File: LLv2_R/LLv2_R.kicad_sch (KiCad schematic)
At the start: 12 parts, among them J1 AudioJack4

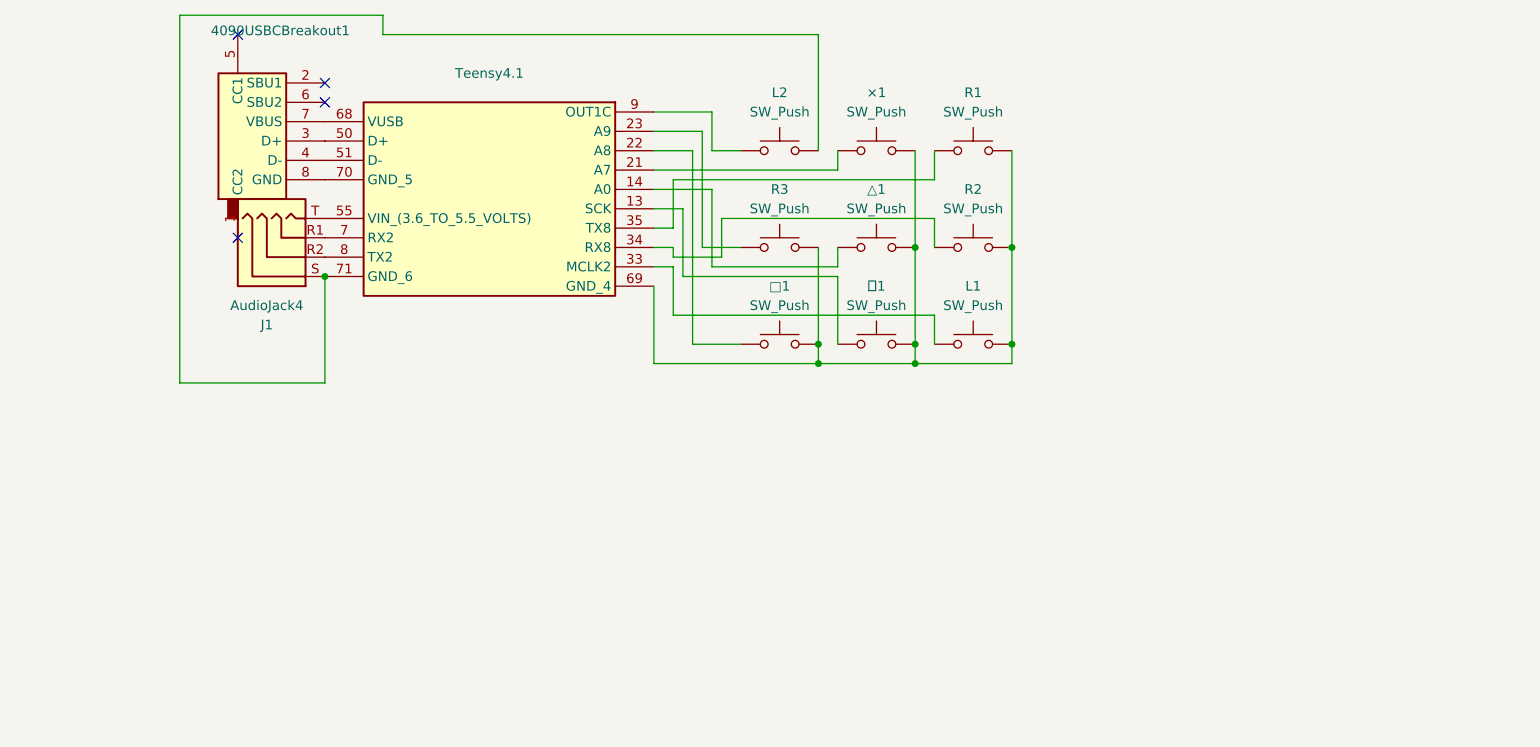
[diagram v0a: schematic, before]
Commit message: Update Softwere
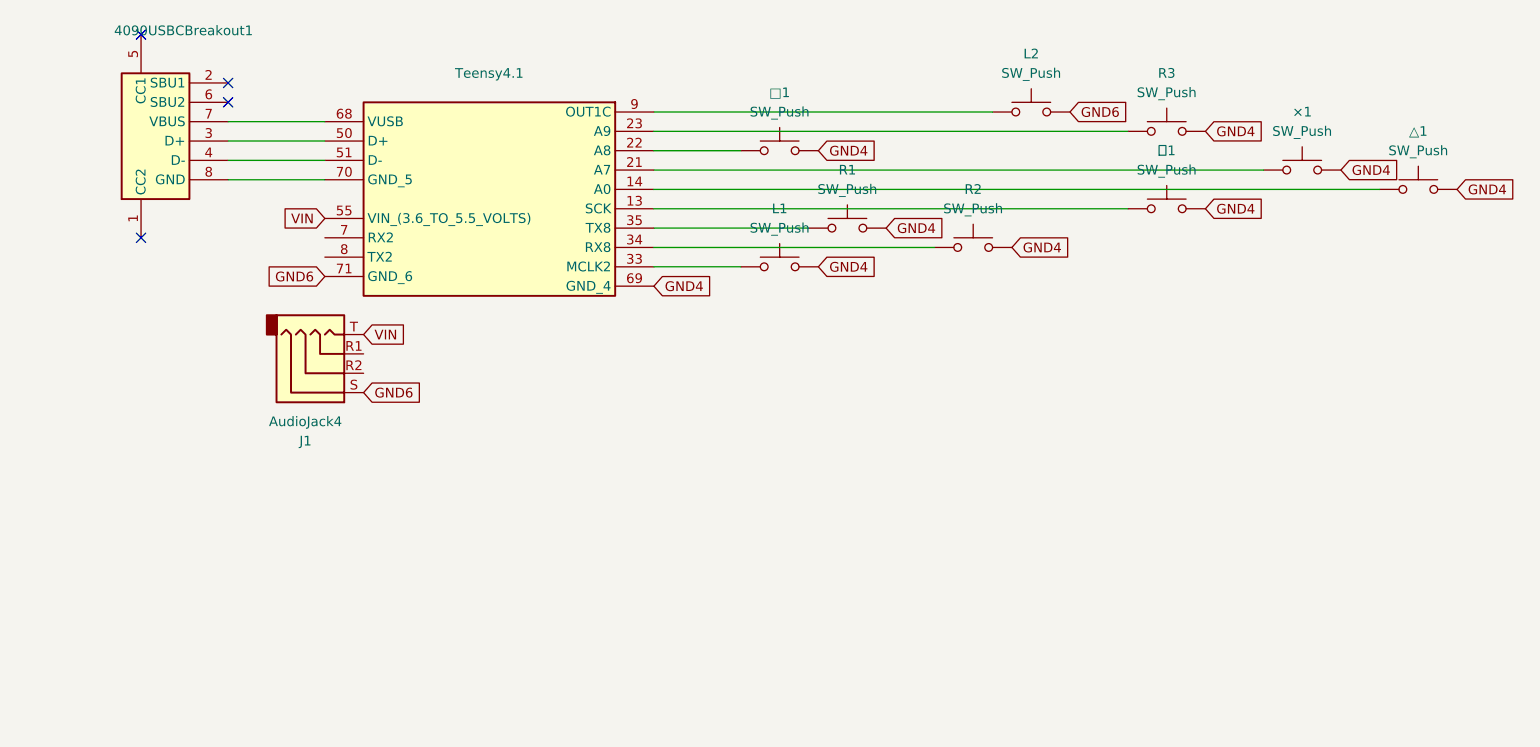
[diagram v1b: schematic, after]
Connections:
- net GND4: now reaches L1.2, R1.2, R2.2, R3.2, Teensy4.1.69 (GND_4), ×1.2, □1.2, △1.2, 〇1.2
- net GND6: now reaches J1.S, L2.2, Teensy4.1.71 (GND_6)
- net at J1.R1: no longer Teensy4.1.7 (RX2)
- net at J1.R2: no longer Teensy4.1.8 (TX2)
- net VIN: now reaches J1.T, Teensy4.1.55 (VIN_(3.6_TO_5.5_VOLTS))
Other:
- moved on the sheet: 4090USBCBreakout1, J1, L1, L2, R1, R3, ×1, □1, △1, 〇1

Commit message: add test script
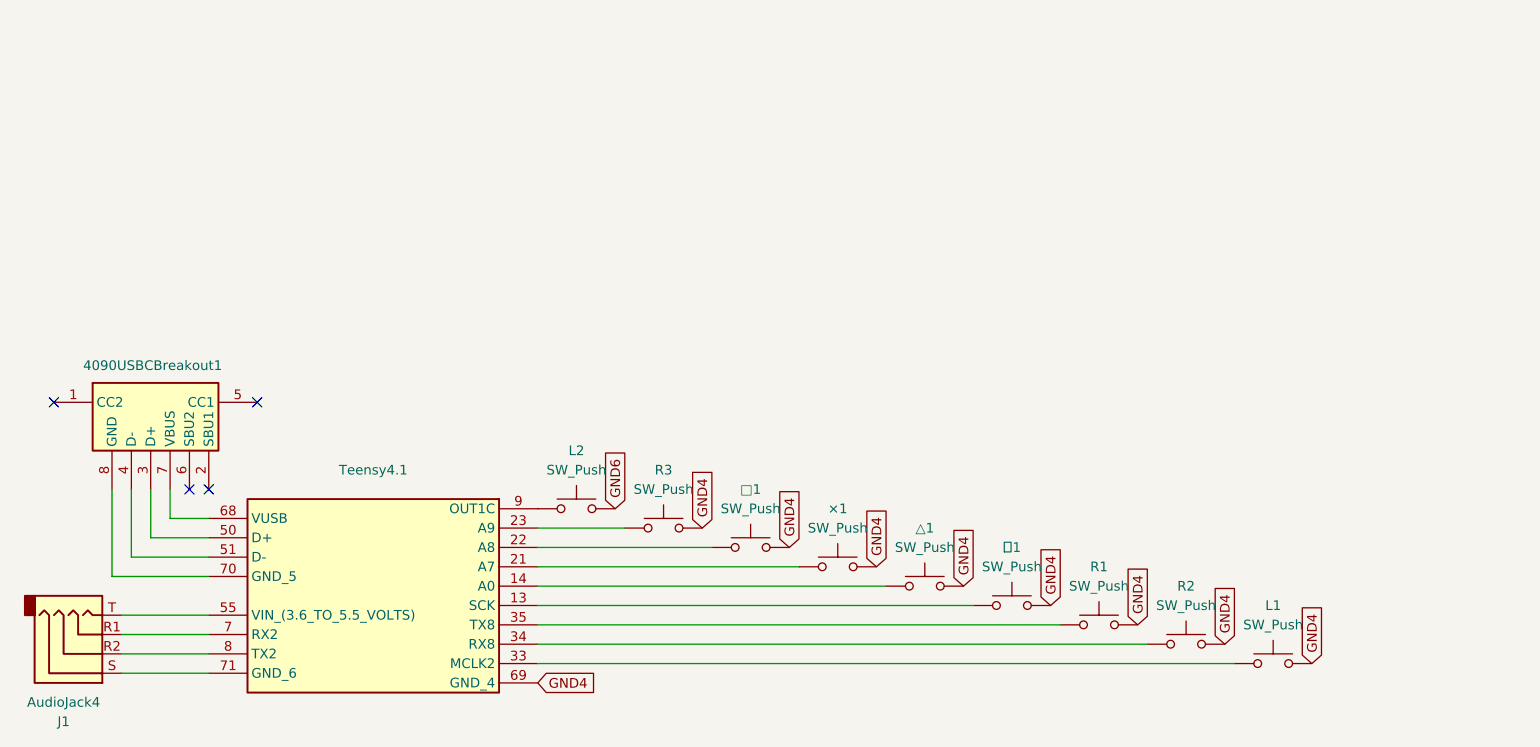
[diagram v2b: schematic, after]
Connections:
- net GND6: no longer J1.S, Teensy4.1.71 (GND_6)
- net at J1.R1: now also Teensy4.1.7 (RX2)
- net at J1.R2: now also Teensy4.1.8 (TX2)
- net VIN: no longer names the net of J1.T, Teensy4.1.55 (VIN_(3.6_TO_5.5_VOLTS))
- new net: J1.S, Teensy4.1.71 (GND_6)
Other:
- moved on the sheet: 4090USBCBreakout1, J1, L1, L2, R1, R2, R3, Teensy4.1, ×1, □1, △1, 〇1
